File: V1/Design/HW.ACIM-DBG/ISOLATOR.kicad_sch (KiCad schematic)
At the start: 23 parts, among them J1 EXT INV DEBUG, J2 Micro USB, J3 PSU DEBUG, J5 INV DEBUG, U1 LOAD SWITCHER, U3 ISO USB 2.0

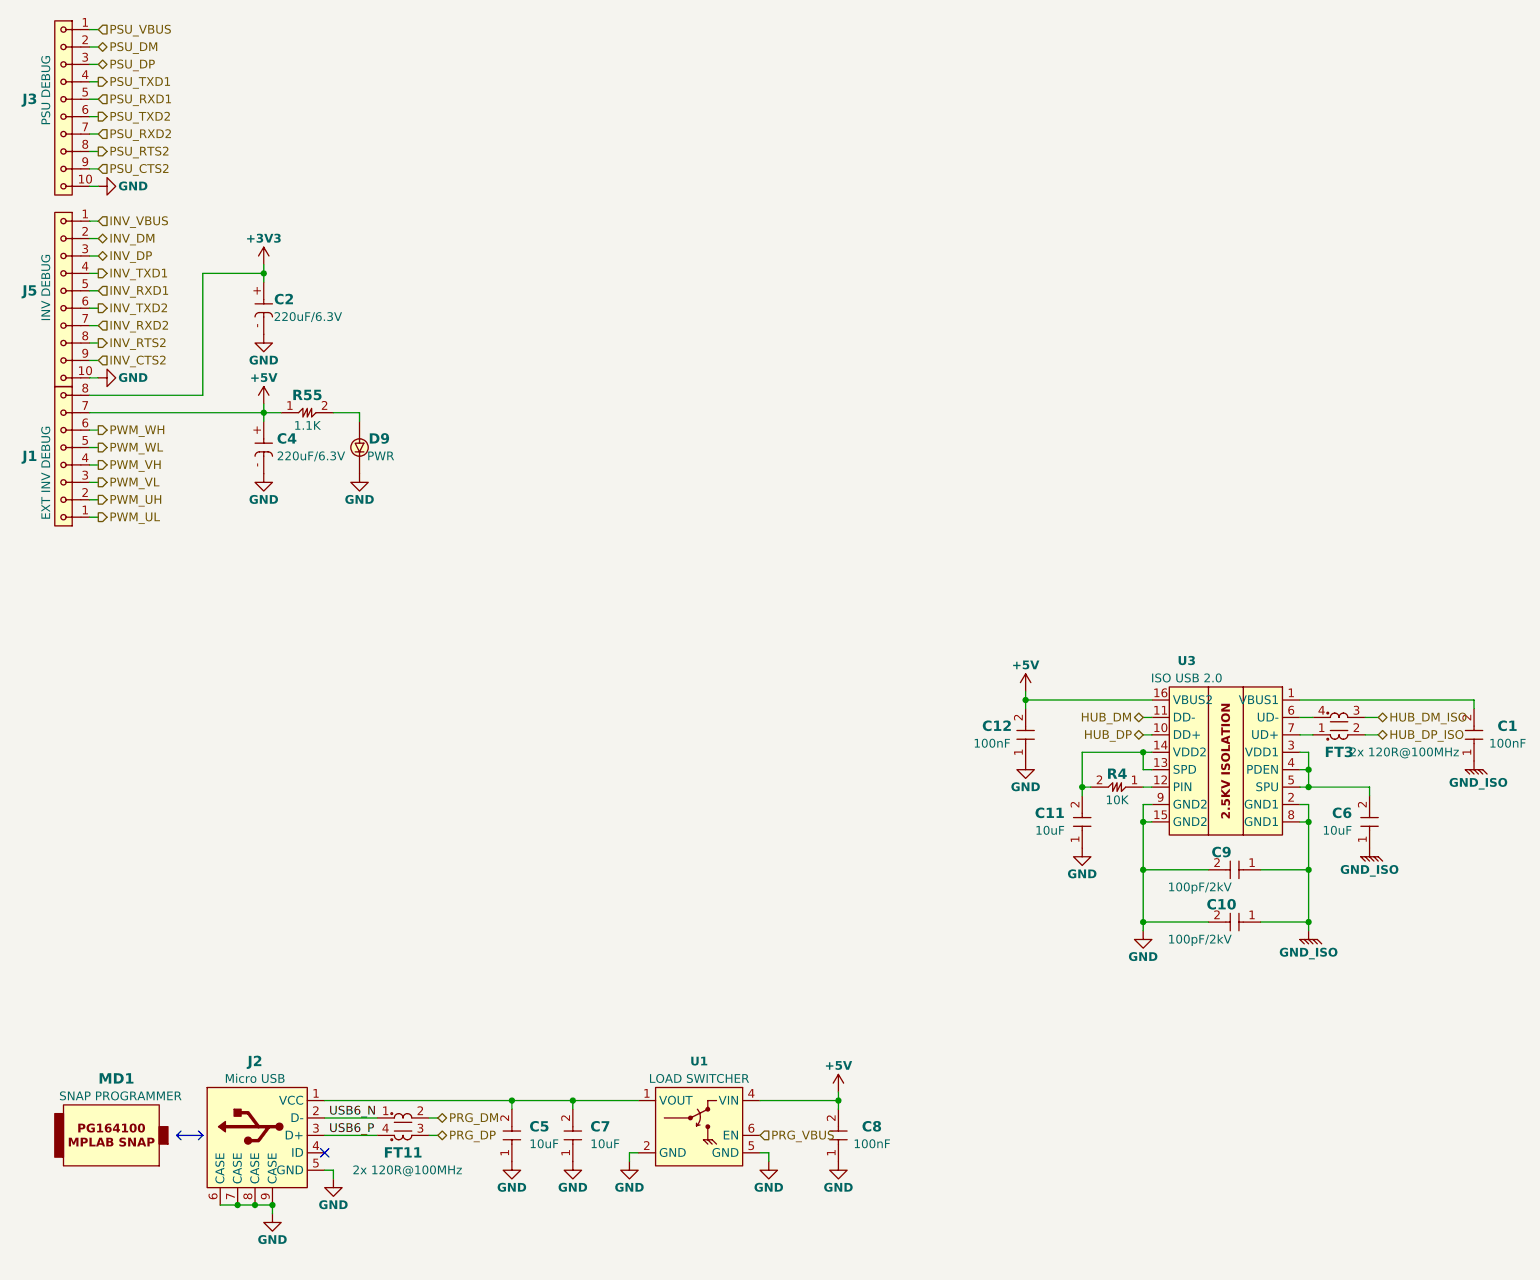
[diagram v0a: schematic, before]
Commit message: V1 schematic update 1
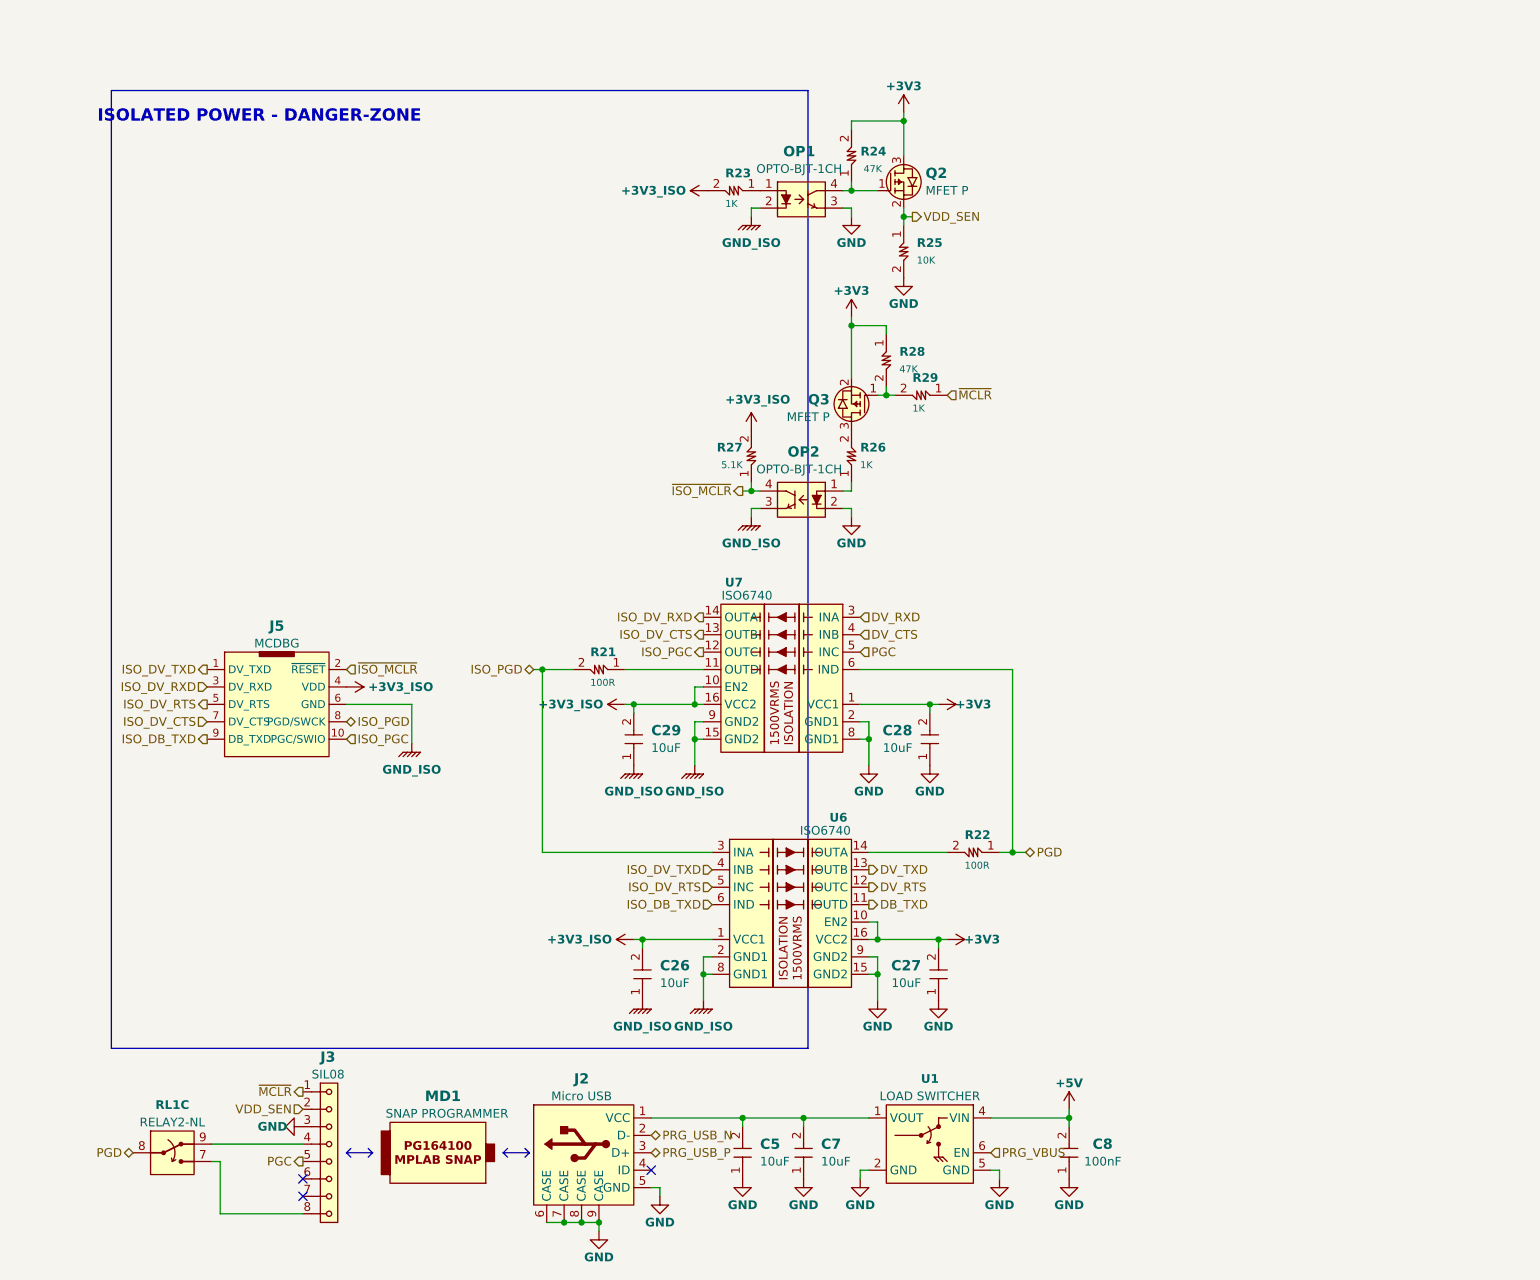
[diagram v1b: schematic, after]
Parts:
- removed C1, C12: 100nF, SAMPI:CAP0603, symbol SAMPI:CERCAP
- removed C10, C9: 100pF/2kV, SAMPI:CAP1206, symbol SAMPI:CERCAP
- removed C11, C6: 10uF, SAMPI:CAP0603, symbol SAMPI:CERCAP
- removed C2, C4: 220uF/6.3V, SAMPI:CAP1411, symbol SAMPI:ELECCAP
- removed D9: PWR, SAMPI:LED0603, symbol SAMPI:WLED
- removed FT11, FT3: 2x 120R@100MHz, SAMPI:IND1210_4P, symbol SAMPI:IND1210_4P
- removed J1: EXT INV DEBUG, SAMPI:HDM1x8x2.54_TH_RA, symbol SAMPI:SIL08
- removed J3: PSU DEBUG, SAMPI:HDF1x10x2.54_TH_RA, symbol SAMPI:SIL10
- removed J5: INV DEBUG, SAMPI:HDF1x10x2.54_TH_RA, symbol SAMPI:SIL10
- removed R4: 10K, SAMPI:RES0603, symbol SAMPI:RES
- removed R55: 1.1K, SAMPI:RES0603, symbol SAMPI:RES
- removed U3: ISO USB 2.0, SAMPI:SOIC16_7.5_AN, symbol SAMPI:ADUM3160
- added C26, C27, C28, C29: 10uF, SAMPI:CAP0603, symbol SAMPI:CERCAP
- added J3: SIL08, symbol SAMPI:SIL08
- added J5: MCDBG, SAMPI:IDC-2x5x2MM-TH, symbol SAMPI:MCDBG
- added OP1, OP2: OPTO-BJT-1CH, SAMPI:OPTO_SO4_7.6MM, symbol SAMPI:OPTO-BJT-1CH
- added Q2, Q3: MFET P, symbol SAMPI:FET_P-CH
- added R21, R22: 100R, Liem:RES0402, symbol SAMPI:RES
- added R23, R26, R29: 1K, Liem:RES0402, symbol SAMPI:RES
- added R24, R28: 47K, Liem:RES0402, symbol SAMPI:RES
- added R25: 10K, Liem:RES0402, symbol SAMPI:RES
- added R27: 5.1K, Liem:RES0402, symbol SAMPI:RES
- added RL1: RELAY2-NL, SAMPI:EA2-5NU, symbol SAMPI:RELAY2-NL
- added U6, U7: ISO6740, SAMPI:SOIC16-W, symbol SAMPI:ISO6740
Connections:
- net +3V3: now also C27.2, C28.2, Q2.3 (D), Q3.2 (S), R24.2, R28.1, U6.10 (EN2), U6.16 (VCC2), U7.1 (VCC1)
- net GND: now also C27.1, C28.1, J3.3, OP1.3 (E), OP2.2 (K), R25.2, U6.15 (GND2), U6.9 (GND2), U7.2 (GND1), U7.8 (GND1)
- net GND_ISO: now also C26.1, C29.1, J5.6 (GND), OP1.2 (K), OP2.3 (E), U6.2 (GND1), U6.8 (GND1), U7.15 (GND2), U7.9 (GND2)
- net USB6_N renamed PRG_USB_N
- net USB6_P renamed PRG_USB_P
- new net: R21.1, U7.11 (OUTD)
- new net: OP1.4 (C), Q2.1 (G), R24.1
- new net: J3.8, RL1.7 (NO2)
- new net: J3.4, RL1.9 (NC2)
- new net: OP1.1 (A), R23.1
- new net: R22.2, U6.14 (OUTA)
- new net: OP2.1 (A), R26.1
- new net: Q3.3 (D), R26.2
- new net: Q3.1 (G), R28.2, R29.2
- new net +3V3_ISO: C26.2, C29.2, J5.4 (VDD), R23.2, R27.2, U6.1 (VCC1), U7.10 (EN2), U7.16 (VCC2)
- new net DB_TXD: U6.11 (OUTD)
- new net DV_CTS: U7.4 (INB)
- new net DV_RTS: U6.12 (OUTC)
- new net DV_RXD: U7.3 (INA)
- new net DV_TXD: U6.13 (OUTB)
- new net ISO_DB_TXD: J5.9 (DB_TXD), U6.6 (IND)
- new net ISO_DV_CTS: J5.7 (DV_CTS), U7.13 (OUTB)
- new net ISO_DV_RTS: J5.5 (DV_RTS), U6.5 (INC)
- new net ISO_DV_RXD: J5.3 (DV_RXD), U7.14 (OUTA)
- new net ISO_DV_TXD: J5.1 (DV_TXD), U6.4 (INB)
- new net ISO_PGC: J5.10 (PGC/SWIO), U7.12 (OUTC)
- new net ISO_PGD: J5.8 (PGD/SWCK), R21.2, U6.3 (INA)
- new net PGC: J3.5, U7.5 (INC)
- new net PGD: R22.1, RL1.8 (COM2), U7.6 (IND)
- new net VDD_SEN: J3.2, Q2.2 (S), R25.1
- new net ~{ISO_MCLR}: J5.2 (~{RESET}), OP2.4 (C), R27.1
- new net ~{MCLR}: J3.1, R29.1
- no-connect marks 1 -> 3
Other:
- note added: "ISOLATED POWER - DANGER-ZONE"
- moved on the sheet: C5, C7, C8, J2, MD1, U1

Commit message: V1 schematic update 2
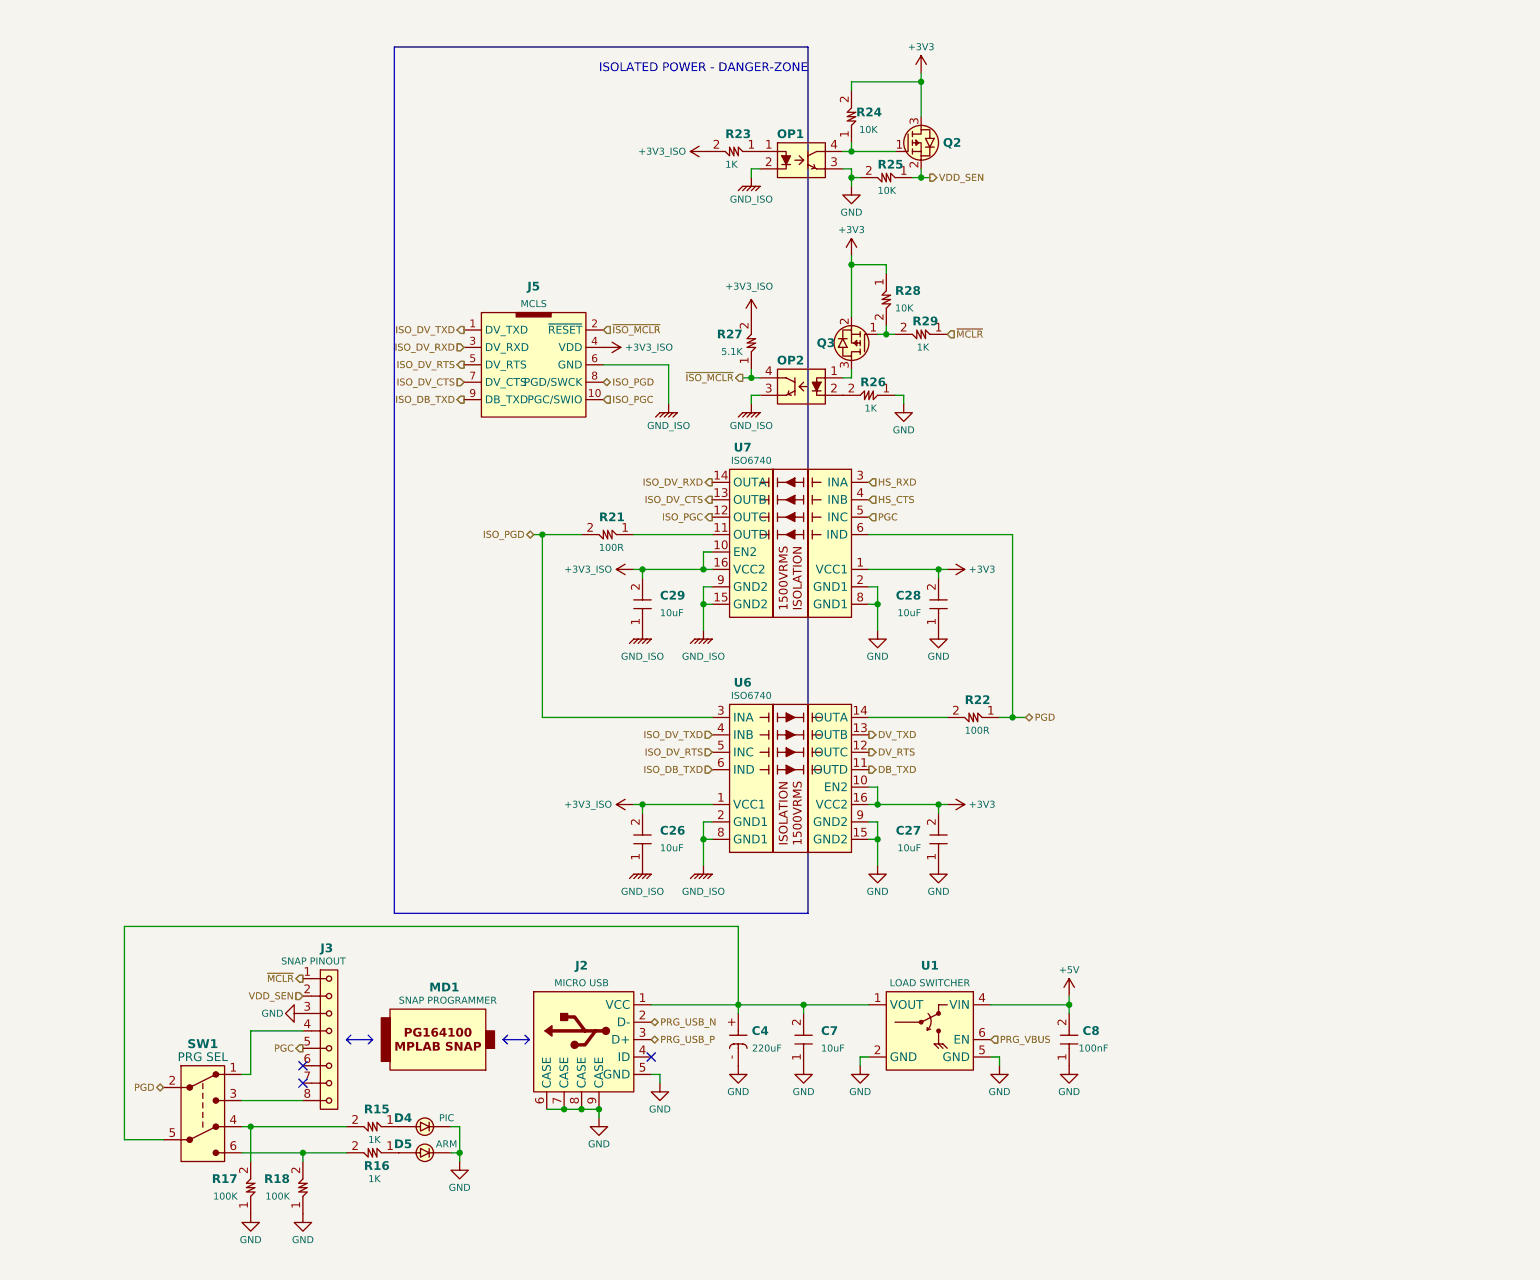
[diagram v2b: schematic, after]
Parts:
- removed C5: 10uF, SAMPI:CAP0603, symbol SAMPI:CERCAP
- removed RL1: RELAY2-NL, SAMPI:EA2-5NU, symbol SAMPI:RELAY2-NL
- added C4: 220uF, Liem:CAP2312-6032, symbol SAMPI:ELECCAP
- added D4: PIC, Liem:LED0603, symbol Liem:RLED
- added D5: ARM, Liem:LED0603, symbol Liem:RLED
- added R15, R16: 1K, Liem:RES0402, symbol SAMPI:RES
- added R17, R18: 100K, Liem:RES0402, symbol SAMPI:RES
- added SW1: PRG SEL, SAMPI:SW_PUSH_2DPDT, symbol SAMPI:SW_DPDT
- C7: Checked OK -> (none); Unit Price 0.079 -> (none)
- C8: Checked OK -> (none); Unit Price 0.0146 -> (none)
- J2: value Micro USB -> MICRO USB; Checked OK -> (none)
- J3: value SIL08 -> SNAP PINOUT; footprint (none) -> SAMPI:HDF1x8x2.54_TH_RA; MFT (none) -> Sullins Connector Solutions; MNP (none) -> PPTC081LGBN-RC
- J5: value MCDBG -> MCLS
- MD1: Checked OK -> (none)
- Q2, Q3: value MFET P -> 20V/2.3A; MFT (none) -> Vishay; MNP (none) -> SI2301DS
- R24, R28: value 47K -> 10K
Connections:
- net GND: now also R26.1, C4.-, D4.K, D5.K, R17.1, R18.1; no longer OP2.2 (K)
- net PGD: now also SW1.2 (COM1)
- net at C7.2, J2.1 (VCC), U1.1 (VOUT): now also C4.+, SW1.5 (COM2)
- net at J3.8: now also SW1.3 (NO1)
- net at J3.4: now also SW1.1 (NC1)
- net at OP2.1 (A): now also Q3.3 (D); no longer R26.1
- net at R26.2: now also OP2.2 (K); no longer Q3.3 (D)
- net DV_CTS renamed HS_CTS
- net DV_RXD renamed HS_RXD
- new net: R15.2, R17.2, SW1.4 (NC2)
- new net: D4.A, R15.1
- new net: R16.2, R18.2, SW1.6 (NO2)
- new net: D5.A, R16.1
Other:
- moved on the sheet: C26, C27, C28, C29, C7, C8, J2, J3, J5, MD1, OP1, OP2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
